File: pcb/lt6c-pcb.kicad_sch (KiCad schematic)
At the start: 19 parts, among them SW1 SW_Push, SW2 SW_Push, SW3 SW_Push, SW4 SW_Push, SW5 SW_Push, SW6 SW_Push, U1 XIAO-RP2040, U2 TPS76318, U3 PMW3360DM-T2QU

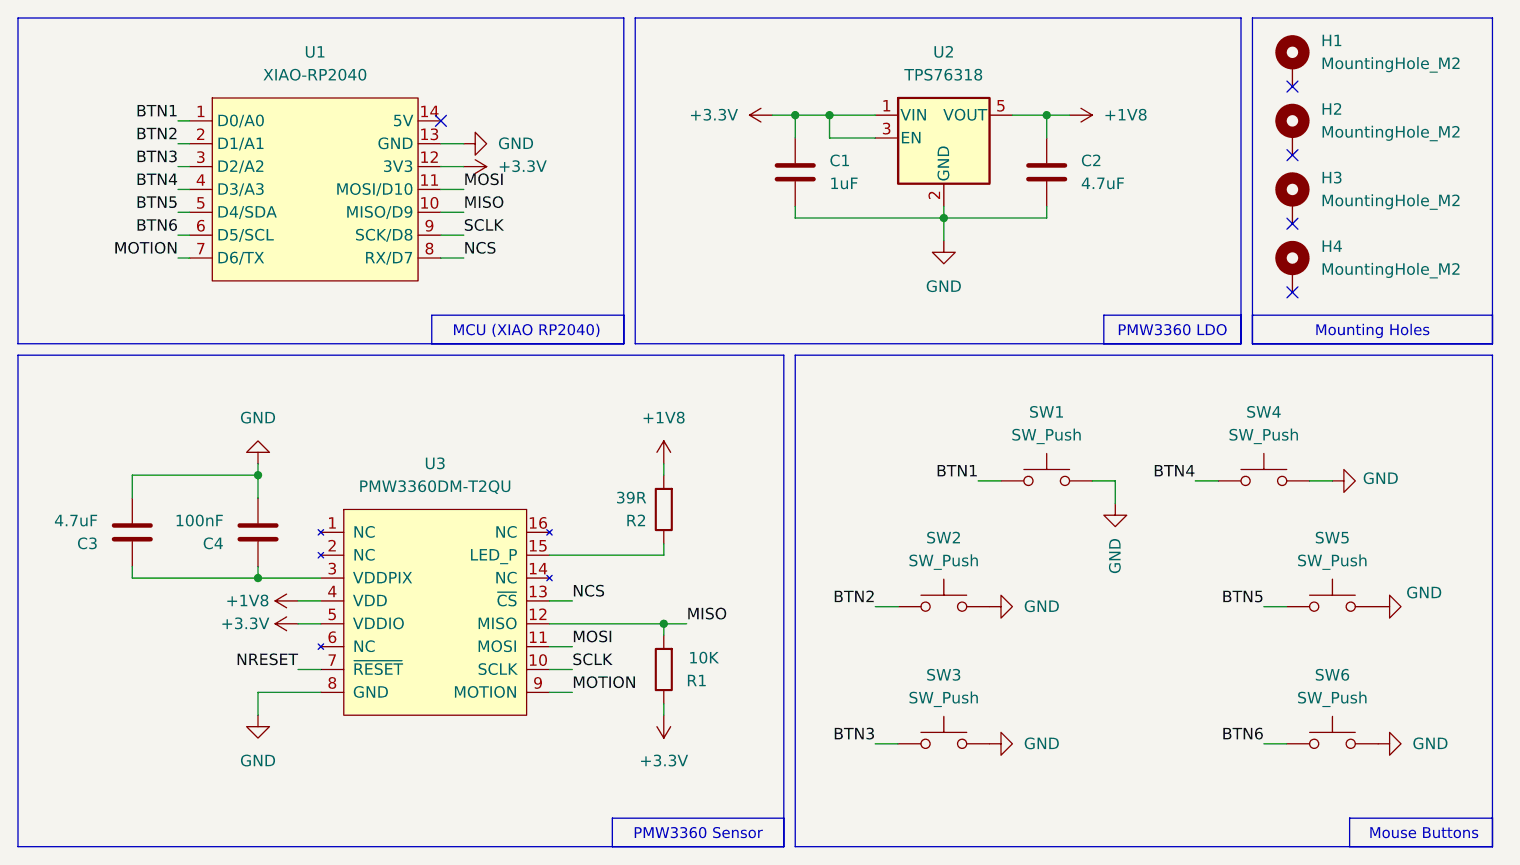
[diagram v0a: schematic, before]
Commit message: Update README.md & .gitattributes
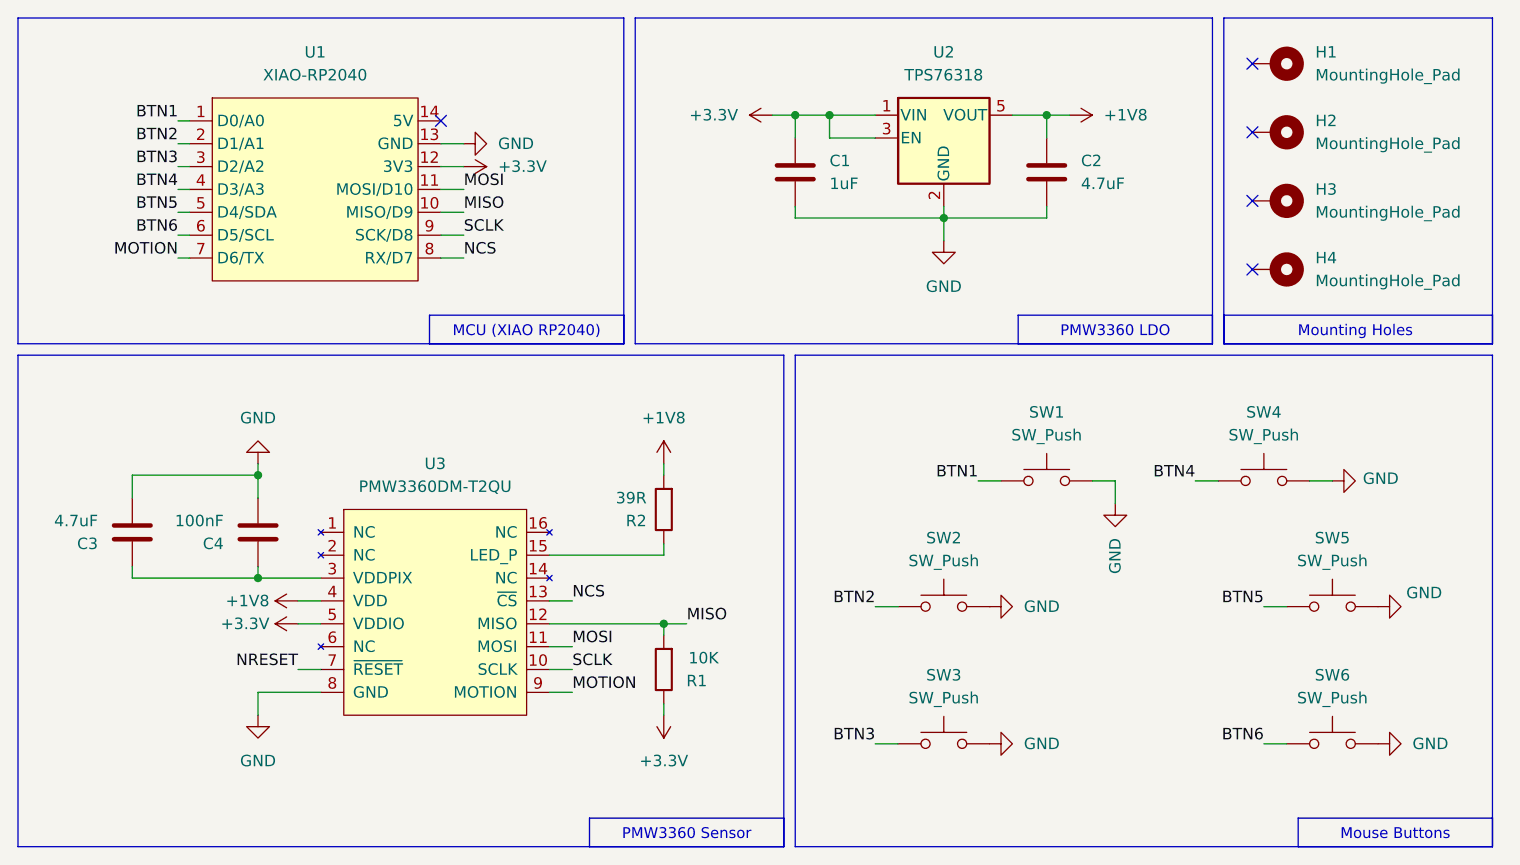
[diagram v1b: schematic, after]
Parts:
- H1, H2, H3, H4: value MountingHole_M2 -> MountingHole_Pad
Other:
- moved on the sheet: H1, H2, H3, H4
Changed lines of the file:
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@@
 	)
 	(no_connect
-		(at 155.575 21.59)
+		(at 151.13 19.05)
 	)
 	(no_connect
-		(at 155.575 29.21)
+		(at 151.13 26.67)
 	)
 	(no_connect
-		(at 155.575 44.45)
+		(at 151.13 41.91)
 	)
 	(no_connect
@@
 	)
 	(no_connect
-		(at 155.575 36.83)
+		(at 151.13 34.29)
 	)
 	(wire
@@
 	)
 	(rectangle
-		(start 151.13 46.99)
+		(start 147.955 46.99)
 		(end 177.8 50.165)
 		(stroke
@@
 	)
 	(rectangle
-		(start 100.33 51.435)
-		(end 177.8 106.045)
+		(start 59.69 46.99)
+		(end 81.28 50.165)
 		(stroke
 			(width 0)
@@
 	)
 	(rectangle
-		(start 59.944 46.99)
-		(end 81.28 50.165)
+		(start 77.47 102.87)
+		(end 99.06 106.045)
 		(stroke
 			(width 0)
@@
 	)
 	(rectangle
-		(start 82.55 13.97)
-		(end 149.86 50.165)
+		(start 100.33 51.435)
+		(end 177.8 106.045)
 		(stroke
 			(width 0)
@@
 	)
 	(rectangle
-		(start 151.13 13.97)
-		(end 177.8 50.165)
+		(start 156.21 102.87)
+		(end 177.8 106.045)
 		(stroke
 			(width 0)
@@
 	)
 	(rectangle
-		(start 161.925 102.87)
-		(end 177.8 106.045)
+		(start 82.55 13.97)
+		(end 146.685 50.165)
 		(stroke
 			(width 0)
@@
 	)
 	(rectangle
-		(start 134.62 46.99)
-		(end 149.86 50.165)
+		(start 147.955 13.97)
+		(end 177.8 50.165)
 		(stroke
 			(width 0)
@@
 	)
 	(rectangle
-		(start 80.01 102.87)
-		(end 99.06 106.045)
+		(start 125.095 46.99)
+		(end 146.685 50.165)
 		(stroke
 			(width 0)
@@
 	(text "PMW3360 LDO"
 		(exclude_from_sim no)
-		(at 142.24 48.895 0)
+		(at 135.89 48.895 0)
 		(effects
 			(font
@@
 	(text "Mounting Holes"
 		(exclude_from_sim no)
-		(at 164.465 48.895 0)
+		(at 162.56 48.895 0)
 		(effects
 			(font
@@
 	(text "PMW3360 Sensor"
 		(exclude_from_sim no)
-		(at 89.535 104.775 0)
+		(at 88.265 104.775 0)
 		(effects
 			(font
@@
 	(text "Mouse Buttons"
 		(exclude_from_sim no)
-		(at 170.18 104.775 0)
+		(at 167.005 104.775 0)
 		(effects
 			(font
@@
 	(symbol
 		(lib_id "Mechanical:MountingHole_Pad")
-		(at 155.575 19.05 0)
+		(at 153.67 19.05 270)
 		(unit 1)
 		(exclude_from_sim yes)
@@
 		(fields_autoplaced yes)
 		(property "Reference" "H1"
-			(at 158.75 16.5099 0)
+			(at 158.115 17.7799 90)
 			(effects
 				(font
@@
 			)
 		)
-		(property "Value" "MountingHole_M2"
-			(at 158.75 19.0499 0)
+		(property "Value" "MountingHole_Pad"
+			(at 158.115 20.3199 90)
 			(effects
 				(font
@@
 		)
 		(property "Footprint" "MountingHole:MountingHole_2.2mm_M2_ISO14580_Pad"
-			(at 155.575 19.05 0)
+			(at 153.67 19.05 0)
 			(effects
 				(font
@@
 		)
 		(property "Datasheet" "~"
-			(at 155.575 19.05 0)
+			(at 153.67 19.05 0)
 			(effects
 				(font
@@
 		)
 		(property "Description" "Mounting Hole with connection"
-			(at 155.575 19.05 0)
+			(at 153.67 19.05 0)
 			(effects
 				(font
@@
 		)
 		(property "JLC" ""
-			(at 155.575 19.05 0)
+			(at 153.67 19.05 0)
 			(effects
 				(font
@@
 		)
 		(property "JLCPosOffset" ""
-			(at 155.575 19.05 0)
+			(at 153.67 19.05 0)
 			(effects
 				(font
@@
 		)
 		(property "JLCRotOffset" ""
-			(at 155.575 19.05 0)
+			(at 153.67 19.05 0)
 			(effects
 				(font
@@
 		)
 		(property "LCSC" ""
-			(at 155.575 19.05 0)
+			(at 153.67 19.05 0)
 			(effects
 				(font
@@
 	(symbol
 		(lib_id "Mechanical:MountingHole_Pad")
-		(at 155.575 26.67 0)
+		(at 153.67 26.67 270)
 		(unit 1)
 		(exclude_from_sim yes)
@@
 		(fields_autoplaced yes)
 		(property "Reference" "H2"
-			(at 158.75 24.1299 0)
+			(at 158.115 25.3999 90)
 			(effects
 				(font
@@
 			)
 		)
-		(property "Value" "MountingHole_M2"
-			(at 158.75 26.6699 0)
+		(property "Value" "MountingHole_Pad"
+			(at 158.115 27.9399 90)
 			(effects
 				(font
@@
 		)
 		(property "Footprint" "MountingHole:MountingHole_2.2mm_M2_ISO14580_Pad"
-			(at 155.575 26.67 0)
+			(at 153.67 26.67 0)
 			(effects
 				(font
@@
 		)
 		(property "Datasheet" "~"
-			(at 155.575 26.67 0)
+			(at 153.67 26.67 0)
 			(effects
 				(font
@@
 		)
 		(property "Description" "Mounting Hole with connection"
-			(at 155.575 26.67 0)
+			(at 153.67 26.67 0)
 			(effects
 				(font
@@
 		)
 		(property "JLC" ""
-			(at 155.575 26.67 0)
+			(at 153.67 26.67 0)
 			(effects
 				(font
@@
 		)
 		(property "JLCPosOffset" ""
-			(at 155.575 26.67 0)
+			(at 153.67 26.67 0)
 			(effects
 				(font
@@
 		)
 		(property "JLCRotOffset" ""
-			(at 155.575 26.67 0)
+			(at 153.67 26.67 0)
 			(effects
 				(font
@@
 		)
 		(property "LCSC" ""
-			(at 155.575 26.67 0)
+			(at 153.67 26.67 0)
 			(effects
 				(font
@@
 	(symbol
 		(lib_id "Mechanical:MountingHole_Pad")
-		(at 155.575 41.91 0)
+		(at 153.67 41.91 270)
 		(unit 1)
 		(exclude_from_sim yes)
@@
 		(fields_autoplaced yes)
 		(property "Reference" "H4"
-			(at 158.75 39.3699 0)
+			(at 158.115 40.6399 90)
 			(effects
 				(font
@@
 			)
 		)
-		(property "Value" "MountingHole_M2"
-			(at 158.75 41.9099 0)
+		(property "Value" "MountingHole_Pad"
+			(at 158.115 43.1799 90)
 			(effects
 				(font
@@
 		)
 		(property "Footprint" "MountingHole:MountingHole_2.2mm_M2_ISO14580_Pad"
-			(at 155.575 41.91 0)
+			(at 153.67 41.91 0)
 			(effects
 				(font
@@
 		)
 		(property "Datasheet" "~"
-			(at 155.575 41.91 0)
+			(at 153.67 41.91 0)
 			(effects
 				(font
@@
 		)
 		(property "Description" "Mounting Hole with connection"
-			(at 155.575 41.91 0)
+			(at 153.67 41.91 0)
 			(effects
 				(font
@@
 		)
 		(property "JLC" ""
-			(at 155.575 41.91 0)
+			(at 153.67 41.91 0)
 			(effects
 				(font
@@
 		)
 		(property "JLCPosOffset" ""
-			(at 155.575 41.91 0)
+			(at 153.67 41.91 0)
 			(effects
 				(font
@@
 		)
 		(property "JLCRotOffset" ""
-			(at 155.575 41.91 0)
+			(at 153.67 41.91 0)
 			(effects
 				(font
@@
 		)
 		(property "LCSC" ""
-			(at 155.575 41.91 0)
+			(at 153.67 41.91 0)
 			(effects
 				(font
@@
 	(symbol
 		(lib_id "Mechanical:MountingHole_Pad")
-		(at 155.575 34.29 0)
+		(at 153.67 34.29 270)
 		(unit 1)
 		(exclude_from_sim yes)
@@
 		(fields_autoplaced yes)
 		(property "Reference" "H3"
-			(at 158.75 31.7499 0)
+			(at 158.115 33.0199 90)
 			(effects
 				(font
@@
 			)
 		)
-		(property "Value" "MountingHole_M2"
-			(at 158.75 34.2899 0)
+		(property "Value" "MountingHole_Pad"
+			(at 158.115 35.5599 90)
 			(effects
 				(font
@@
 		)
 		(property "Footprint" "MountingHole:MountingHole_2.2mm_M2_ISO14580_Pad"
-			(at 155.575 34.29 0)
+			(at 153.67 34.29 0)
 			(effects
 				(font
@@
 		)
 		(property "Datasheet" "~"
-			(at 155.575 34.29 0)
+			(at 153.67 34.29 0)
 			(effects
 				(font
@@
 		)
 		(property "Description" "Mounting Hole with connection"
-			(at 155.575 34.29 0)
+			(at 153.67 34.29 0)
 			(effects
 				(font
@@
 		)
 		(property "JLC" ""
-			(at 155.575 34.29 0)
+			(at 153.67 34.29 0)
 			(effects
 				(font
@@
 		)
 		(property "JLCPosOffset" ""
-			(at 155.575 34.29 0)
+			(at 153.67 34.29 0)
 			(effects
 				(font
@@
 		)
 		(property "JLCRotOffset" ""
-			(at 155.575 34.29 0)
+			(at 153.67 34.29 0)
 			(effects
 				(font
@@
 		)
 		(property "LCSC" ""
-			(at 155.575 34.29 0)
+			(at 153.67 34.29 0)
 			(effects
 				(font
